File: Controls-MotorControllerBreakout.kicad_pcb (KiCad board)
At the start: 2 copper layers, 48.5 x 34.5 mm, 17 parts, among them J1 MC CAN 1, J2 MC CAN 2, J3 CAN INTRFC, J4 EXT PWR, J5 CANDAPTER, Q1 PMV35EPER

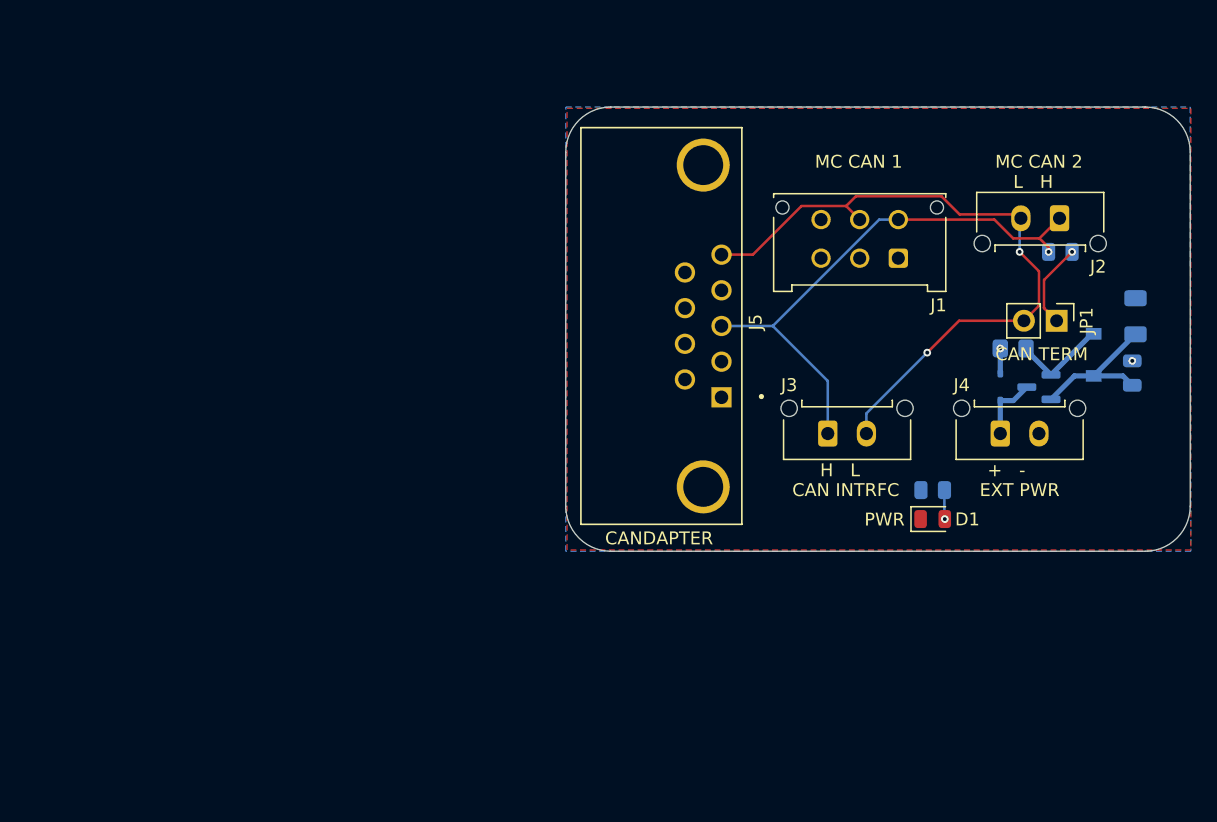
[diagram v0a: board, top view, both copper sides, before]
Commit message: layout kinda screwy but it works?
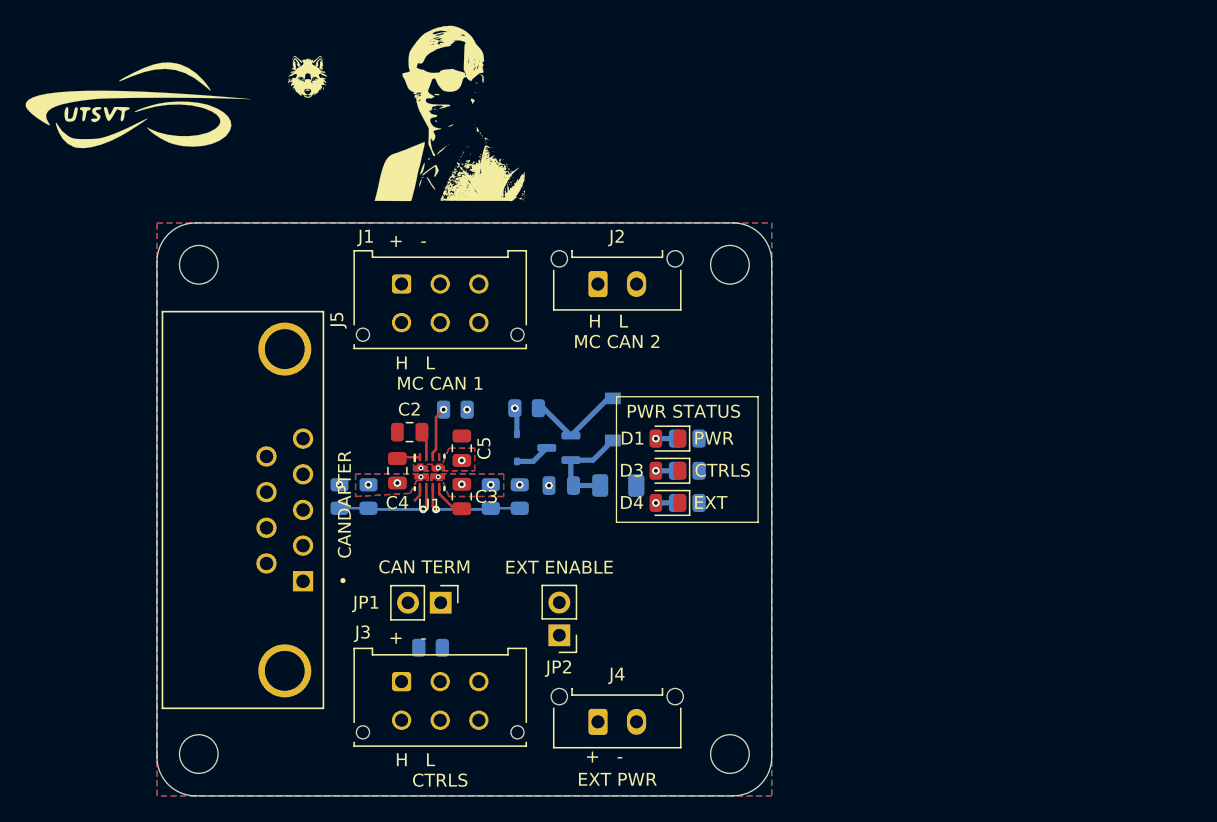
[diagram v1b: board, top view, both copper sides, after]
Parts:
- added C2: 0.1u, Capacitor_SMD:C_0805_2012Metric, F.Cu at (92.1, 60.2)
- added C3: 0.1u, Capacitor_SMD:C_0805_2012Metric, F.Cu at (96.2, 65.2)
- added C4: 0.1u, Capacitor_SMD:C_0805_2012Metric, F.Cu at (91.2, 63.2)
- added C5: 1u, Capacitor_SMD:C_0805_2012Metric, F.Cu at (96.2, 61.5)
- added D3: CTRLS, LED_SMD:LED_0805_2012Metric, F.Cu at (112.2, 63.2)
- added D4: EXT, LED_SMD:LED_0805_2012Metric, F.Cu at (112.2, 65.8)
- added H1: MountingHole, MountingHole:MountingHole_3mm, F.Cu at (75.8, 47.2)
- added H2: MountingHole, MountingHole:MountingHole_3mm, F.Cu at (75.8, 85.2)
- added H3: MountingHole, MountingHole:MountingHole_3mm, F.Cu at (117.0, 85.2)
- added H4: MountingHole, MountingHole:MountingHole_3mm, F.Cu at (117.0, 47.2)
- added JP2: EXT ENABLE, Connector_PinHeader_2.54mm:PinHeader_1x02_P2.54mm_Vertical, F.Cu at (103.8, 76.0)
- added LOGO2: Hallock, UTSVT_Special:Hallock_Image_Tiny, F.Cu at (94.8, 35.3)
- added R10: 22.1k, Resistor_SMD:R_0805_2012Metric, B.Cu at (113.7, 65.8)
- added R4: 100k, Resistor_SMD:R_0805_2012Metric, B.Cu at (95.7, 58.5)
- added R5: 62k, Resistor_SMD:R_0805_2012Metric, B.Cu at (88.9, 65.2)
- added R6: 5k, Resistor_SMD:R_0805_2012Metric, B.Cu at (86.7, 65.2)
- added R7: 5k, Resistor_SMD:R_0805_2012Metric, B.Cu at (100.7, 65.2)
- added R8: 62k, Resistor_SMD:R_0805_2012Metric, B.Cu at (98.4, 65.2)
- added R9: 22.1k, Resistor_SMD:R_0805_2012Metric, B.Cu at (113.7, 63.2)
- added U1: TPS2121RUXR, TPS2121:RUX0012A, F.Cu at (93.7, 63.4)
- G***, LOGO1: moved to F.Cu
- J3: value CAN INTRFC -> CTRLS; footprint Connector_Molex:Molex_Micro-Fit_3.0_43650-0215_1x02_P3.00mm_Vertical -> Connector_Molex:Molex_Micro-Fit_3.0_43045-0612_2x03_P3.00mm_Vertical
- R3: footprint Resistor_SMD:R_0805_2012Metric_Pad1.20x1.40mm_HandSolder -> Resistor_SMD:R_0805_2012Metric
- moved R1 57.8 mm to (93.8, 77.0)
- moved G*** 53.6 mm to (84.2, 32.8), turned to 0 degrees
- moved JP1 52.6 mm to (94.5, 73.5)
- moved C1 45.2 mm to (103.9, 64.4), turned to 180 degrees
- moved F1 42.3 mm to (108.3, 64.4), turned to 0 degrees
- moved LOGO1 41.6 mm to (70.8, 35.0), turned to 0 degrees
- moved J1 38.6 mm to (91.5, 48.7), turned to 0 degrees
- moved J4 38.4 mm to (106.8, 82.8)
- moved J3 38.3 mm to (91.5, 79.6)
- moved R3 38.1 mm to (101.2, 58.4)
- moved D2 37.8 mm to (100.5, 61.5)
- moved Z1 37.7 mm to (107.9, 59.3)
- moved Q1 37.6 mm to (103.7, 61.5)
- moved J2 36.2 mm to (106.8, 48.8), turned to 0 degrees
- moved J5 35.5 mm to (82.4, 66.3)
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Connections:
- D2 pad 2: /EXT_PWR -> /PowerDist/+12V_SEL
- J3 pad 1: /CAN_H -> /+12V_CTRLS
- J3 pad 2: /CAN_L -> GND
- J4 pad 1: /EXT_PWR -> /+12V_EXT
- Q1 pad 3: /EXT_PWR -> /PowerDist/+12V_SEL
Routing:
- net /CAN_L: track 53.2 -> 0.00 mm, vias 2 -> 0
- net /CAN_H: track 42.4 -> 0.00 mm, vias 1 -> 0
- net /PowerDist/OV2: track 0.00 -> 8.39 mm, vias 0 -> 1
- net /PowerDist/OV1: track 0.00 -> 8.39 mm, vias 0 -> 1
- net Net-(JP1-A): track 6.66 -> 0.00 mm, vias 1 -> 0
- net GND: track 1.95 -> 8.43 mm, vias 2 -> 5
- net /EXT_PWR: track 5.06 -> 0.00 mm
- net /PowerDist/ILM: track 0.00 -> 4.05 mm, vias 0 -> 1
- net Net-(Q1-S): track 12.0 -> 8.01 mm
- net /PowerDist/+12V_SEL: track 0.00 -> 2.75 mm, vias 0 -> 3
- net /PowerDist/CSS: track 0.00 -> 2.09 mm
- net Net-(D4-A): track 0.00 -> 1.53 mm, vias 0 -> 1
- net Net-(D3-A): track 0.00 -> 1.53 mm, vias 0 -> 1
- net Net-(D1-A): track 2.32 -> 1.53 mm
- net /PowerDist/+12V_EXT_EN: vias 0 -> 3
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- added copper zone on B.Cu, net /+12V_CTRLS
- added copper zone on F.Cu, net /+12V_CTRLS
- added copper zone on B.Cu, net /PowerDist/+12V_EXT_EN
- added copper zone on F.Cu, net /PowerDist/+12V_EXT_EN
- added copper zone on B.Cu, net /PowerDist/+12V_SEL
- added copper zone on F.Cu, net /PowerDist/+12V_SEL
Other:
- board size 48.5 x 34.5 mm -> 47.8 x 44.5 mm
- board text added: "PWR STATUS"
- board text added: "TODO: add back all useful labels and stuff from v1"
- board text removed: "L H"
- board text removed: "Motor Controller Breakout"
- board text removed: "PWR"
- board text removed: "Ravi Shah 2024"
- board text removed: "profinity/controls pls work :)"
